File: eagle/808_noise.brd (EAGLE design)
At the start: 100 x 82.5 mm, 25 parts, among them IC1 TL072P, Q1 2N3904

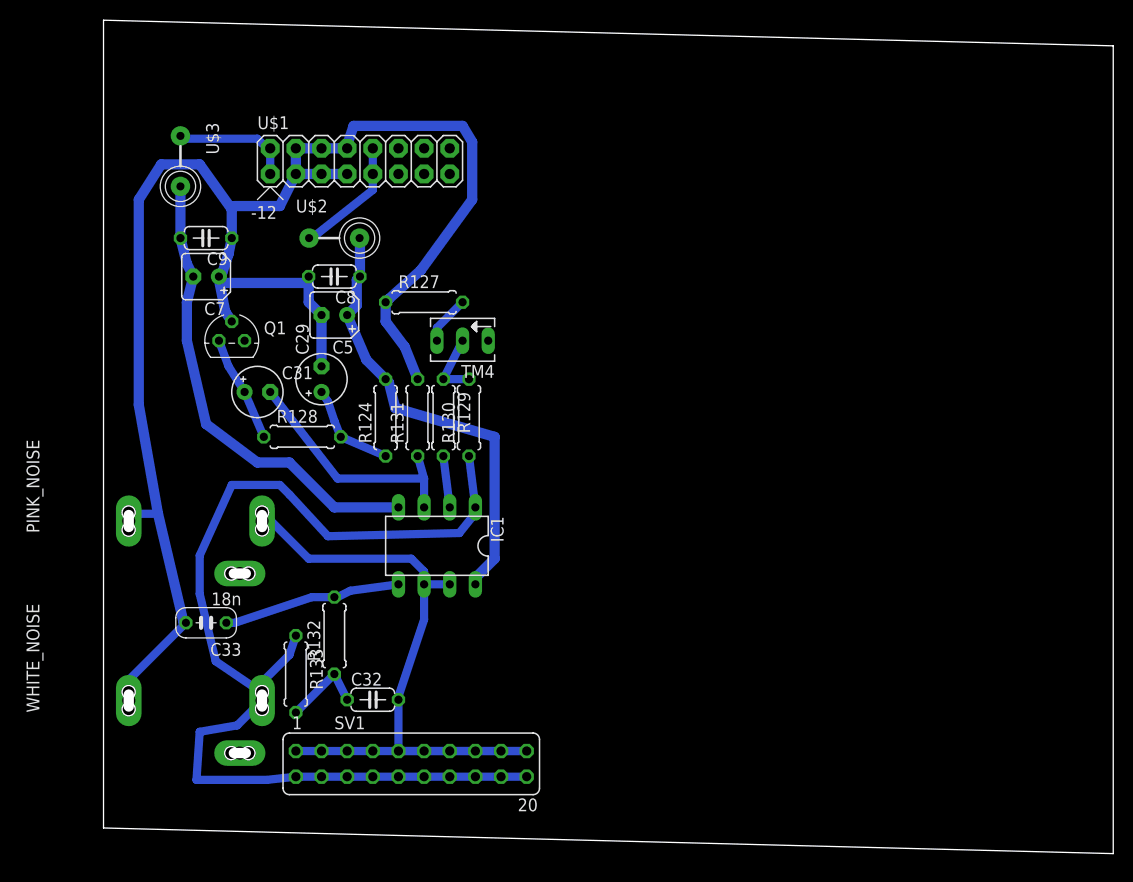
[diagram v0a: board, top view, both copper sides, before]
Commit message: cutout
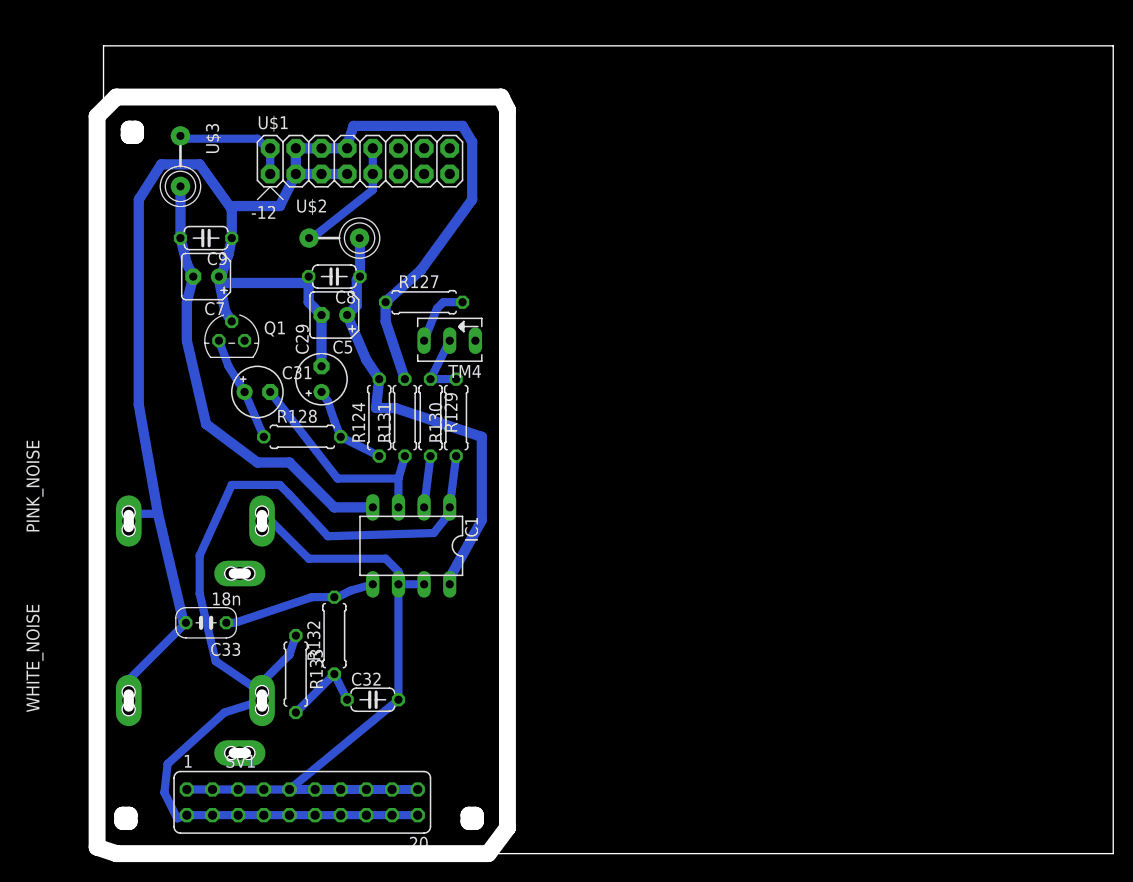
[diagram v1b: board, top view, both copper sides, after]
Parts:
- moved SV1 11.4 mm to (19.7, 5.08)
- moved IC1 2.54 mm to (30.5, 30.5)
- moved R129 1.27 mm to (32.4, 43.2)
- moved R130 1.27 mm to (34.9, 43.2)
- moved TM4 1.27 mm to (34.3, 50.8)
- moved R131 1.27 mm to (29.8, 43.2)
- moved R124 0.64 mm to (27.3, 43.2)
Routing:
- net WN: track 109.0 -> 102.7 mm
- net PN: track 74.4 -> 80.4 mm
- net N$280: track 24.6 -> 22.1 mm
- net -15V: track 46.2 -> 43.7 mm
- net N$494: track 17.7 -> 15.2 mm
- net N$228: track 4.86 -> 6.22 mm
- net N$492: track 9.70 -> 9.12 mm
- net GND: track 163.3 -> 162.8 mm
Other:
- board size 100 x 82.5 mm -> 100.6 x 80 mm
